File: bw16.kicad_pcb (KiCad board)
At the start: 2 copper layers, 30.8 x 57 mm, 28 parts, among them J1 Conn_01x08_Male, J2 Conn_01x08_Male, J6 +3V3, J7 GND, J8 VIN, J9 Conn_01x06_Male, M1 BW16, SW1 RESET, SW2 BURN, U1 AP1117-33

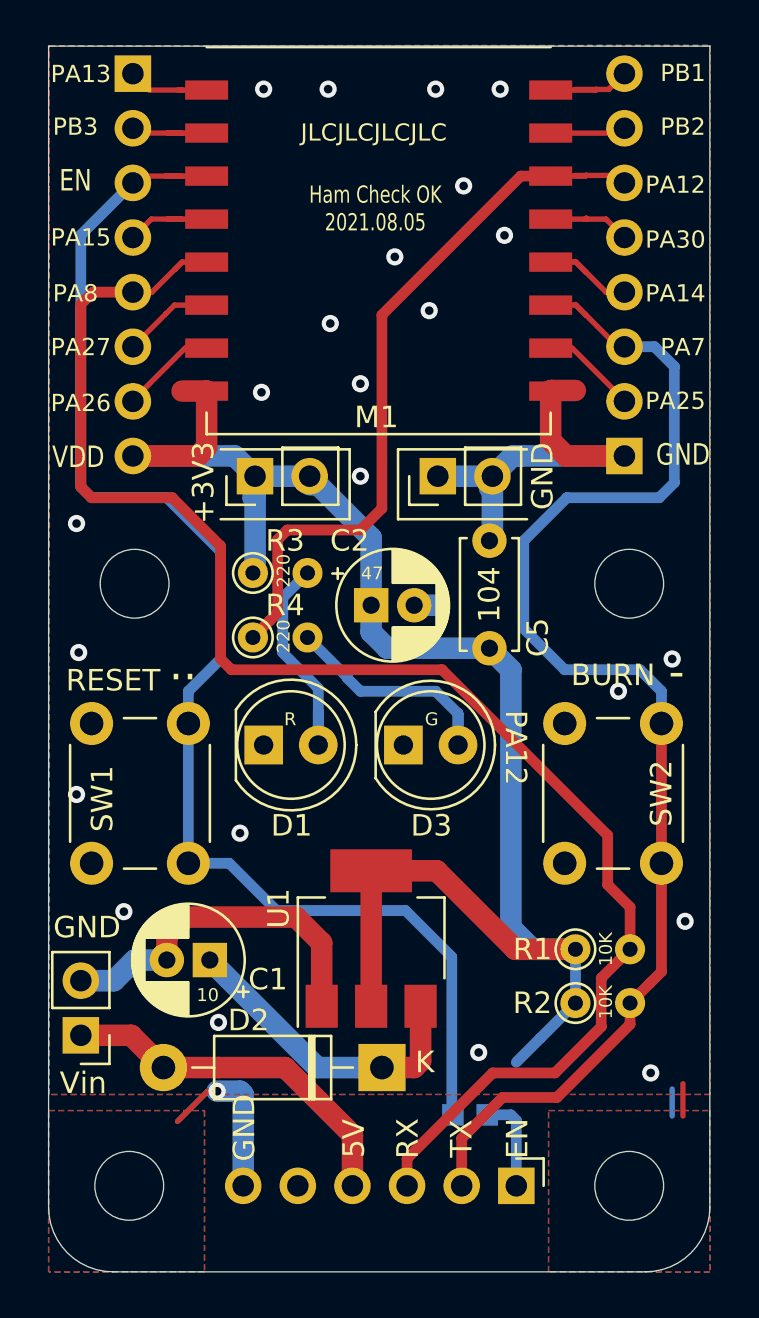
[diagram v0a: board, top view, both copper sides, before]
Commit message: Add files via upload
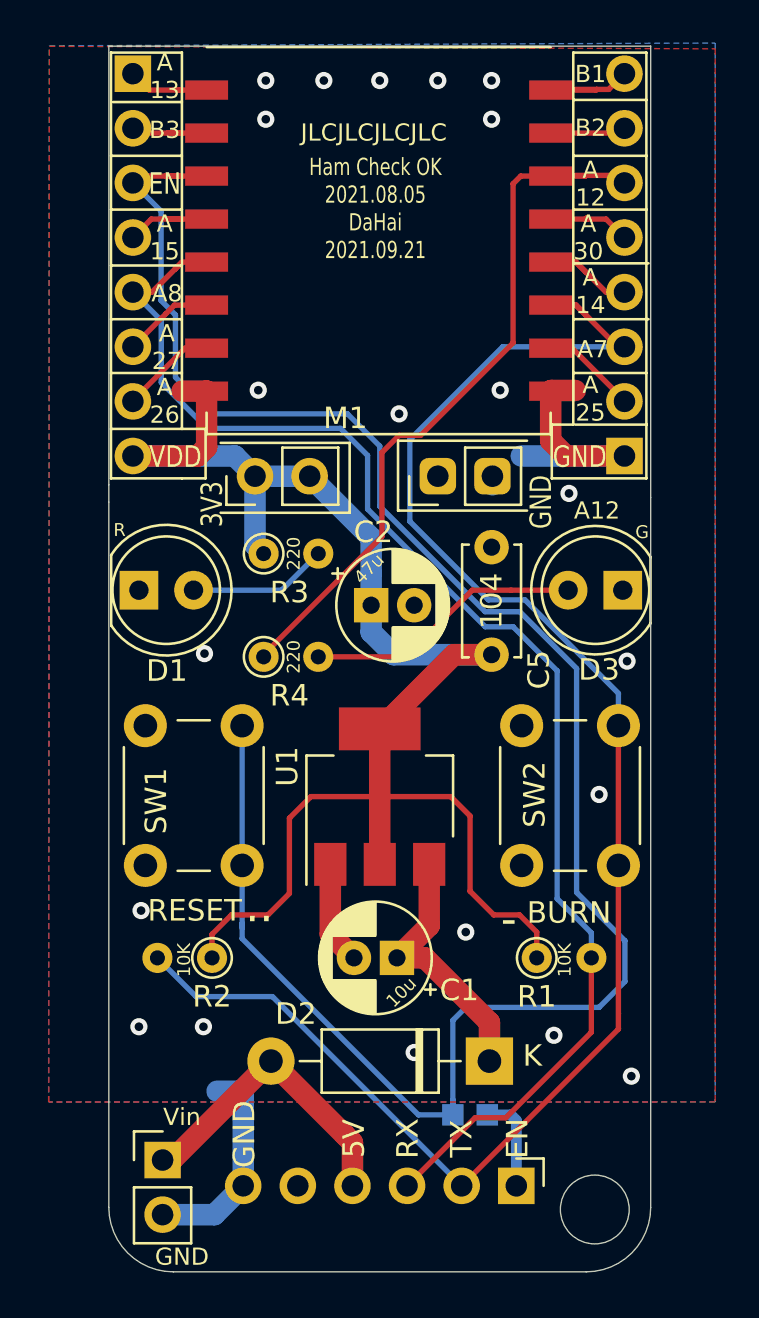
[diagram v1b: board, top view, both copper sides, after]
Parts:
- removed G2: qrcode, pcb:Untitled
- removed H1, H2, H3: MountingHole, MountingHole:MountingHole_3.2mm_M3
- J6: value +3V3 -> 3V3
- moved R2 17.0 mm to (125.6, 122.4), turned to 180 degrees
- moved D3 12.5 mm to (144.7, 105.3), turned to 180 degrees
- moved D1 9.25 mm to (122.2, 105.3)
- moved C1 8.70 mm to (134.2, 122.4)
- moved J8 6.93 mm to (123.3, 131.8), turned to 0 degrees
- moved U1 6.61 mm to (133.4, 114.9)
- moved D2 5.01 mm to (138.5, 127.2)
- moved SW1 2.50 mm to (122.5, 118.1)
- moved SW2 2.00 mm to (140.0, 118.1)
- moved H4 1.94 mm to (143.4, 134.1)
- moved R1 1.84 mm to (140.7, 122.4)
- moved R3 1.03 mm to (128.0, 103.6)
- moved R4 1.03 mm to (128.0, 108.4)
- moved C5 0.32 mm to (138.6, 108.3)
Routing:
- net /EN: track 64.0 -> 93.0 mm
- net /GND: track 50.6 -> 27.0 mm, vias 24 -> 21
- net /LOG_TX: track 61.2 -> 78.0 mm
- net /LOG_RX: track 72.6 -> 63.6 mm
- net /VDD33: track 80.1 -> 73.9 mm
- net Net-(D1-Pad2): track 10.2 -> 6.50 mm
- net /VIN: track 16.9 -> 14.3 mm
- net Net-(C1-Pad1): track 14.5 -> 12.3 mm
- net Net-(D3-Pad2): track 10.9 -> 12.9 mm
- net /PA12: track 34.1 -> 33.5 mm
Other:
- board size 30.8 x 57 mm -> 25.2 x 57 mm
- board text added: "10u"
- board text added: "47u"
- board text added: "A 12"
- board text added: "A 13"
- board text added: "A 14"
- board text added: "A 15"
- board text added: "A 25"
- board text added: "A 26"
- board text added: "A 27"
- board text added: "A 30"
- board text added: "A12"
- board text added: "A7"
- board text added: "A8"
- board text added: "B1"
- board text added: "B2"
- board text added: "B3"
- board text added: "Ham Check OK 2021.08.05 DaHai 2021.09.21"
- board text removed: "10"
- board text removed: "47"
- board text removed: "Ham Check OK 2021.08.05"
- board text removed: "PA12"
- board text removed: "PA13"
- board text removed: "PA14"
- board text removed: "PA15"
- board text removed: "PA25"
- board text removed: "PA26"
- board text removed: "PA27"
- board text removed: "PA30"
- board text removed: "PA7"
- board text removed: "PA8"
- board text removed: "PB1"
- board text removed: "PB2"
- board text removed: "PB3"
